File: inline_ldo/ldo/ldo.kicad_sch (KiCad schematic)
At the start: 14 parts, among them J2 USB_A, U2 LT3045xDD

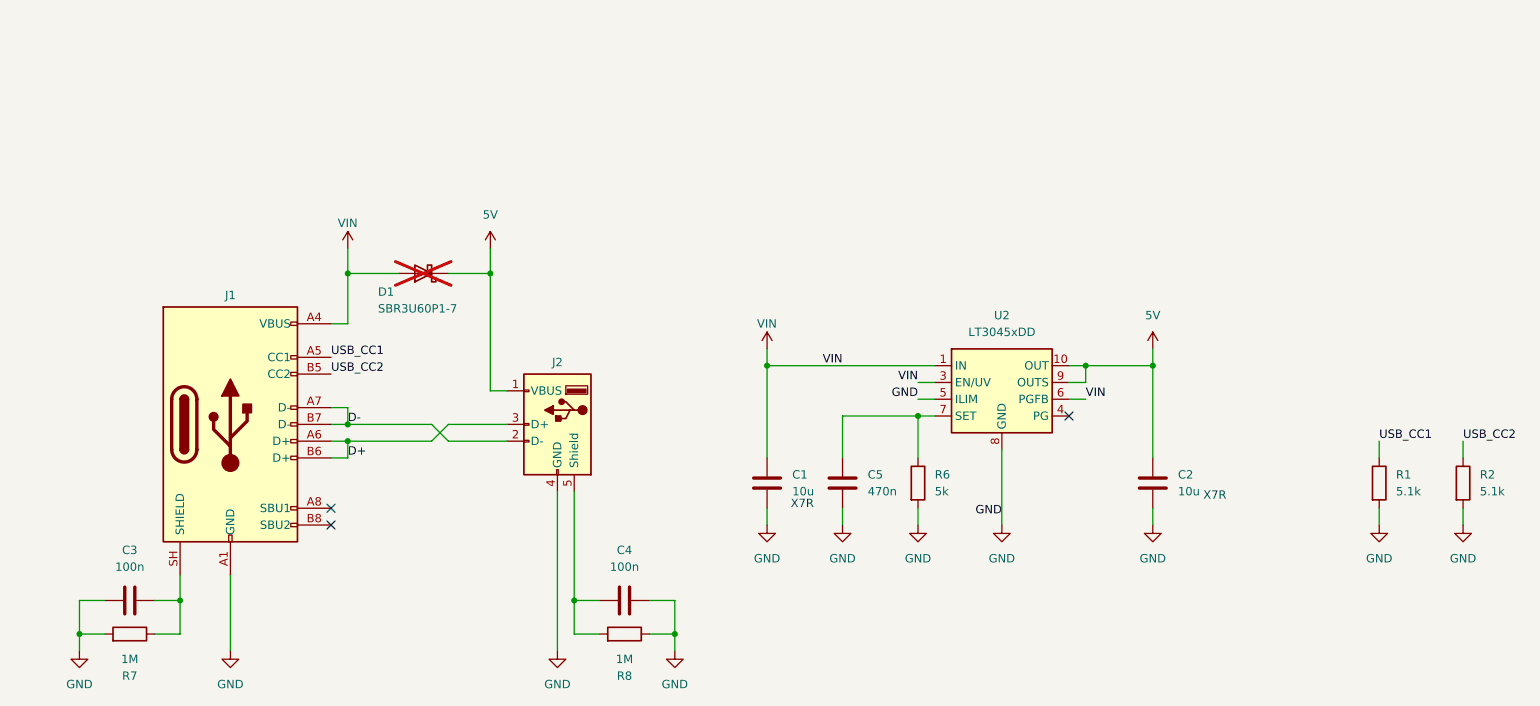
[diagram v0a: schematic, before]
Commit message: minor
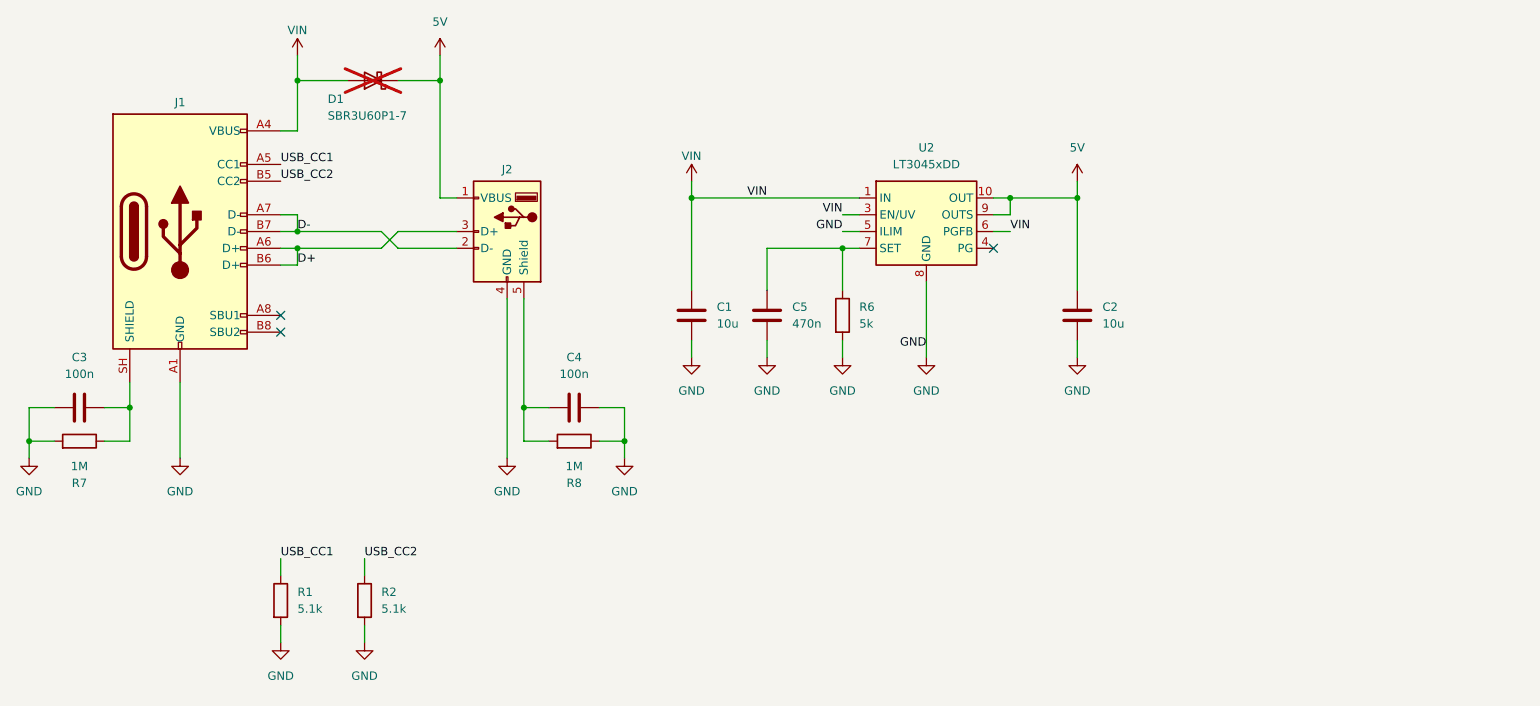
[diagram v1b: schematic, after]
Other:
- note removed: "X7R"
- moved on the sheet: C1, C2, C3, C4, C5, D1, J1, J2, R1, R2, R6, R7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
